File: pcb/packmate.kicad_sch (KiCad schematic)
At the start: 14 parts, among them Q1 2N7002E, SW2 Reset Button, SW3 Left Button, SW4 Right Button, SW6 Wireless On/Off Switch

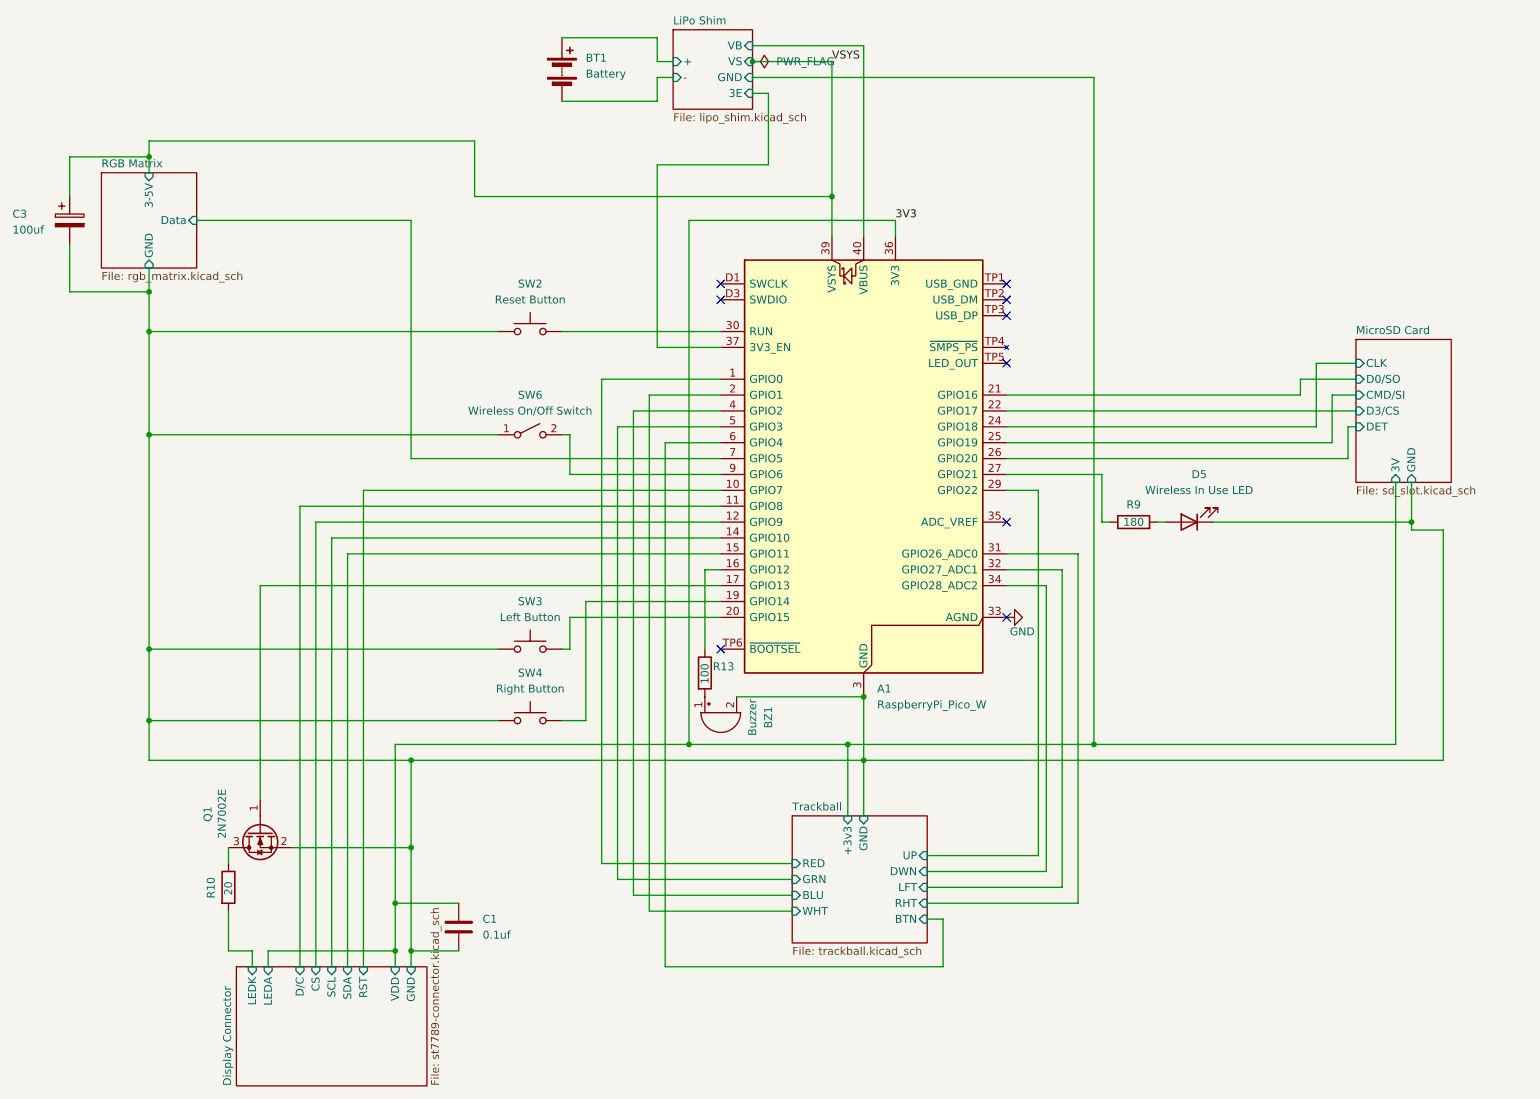
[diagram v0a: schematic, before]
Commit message: Still improving pcb, I learned what a fiducial is today
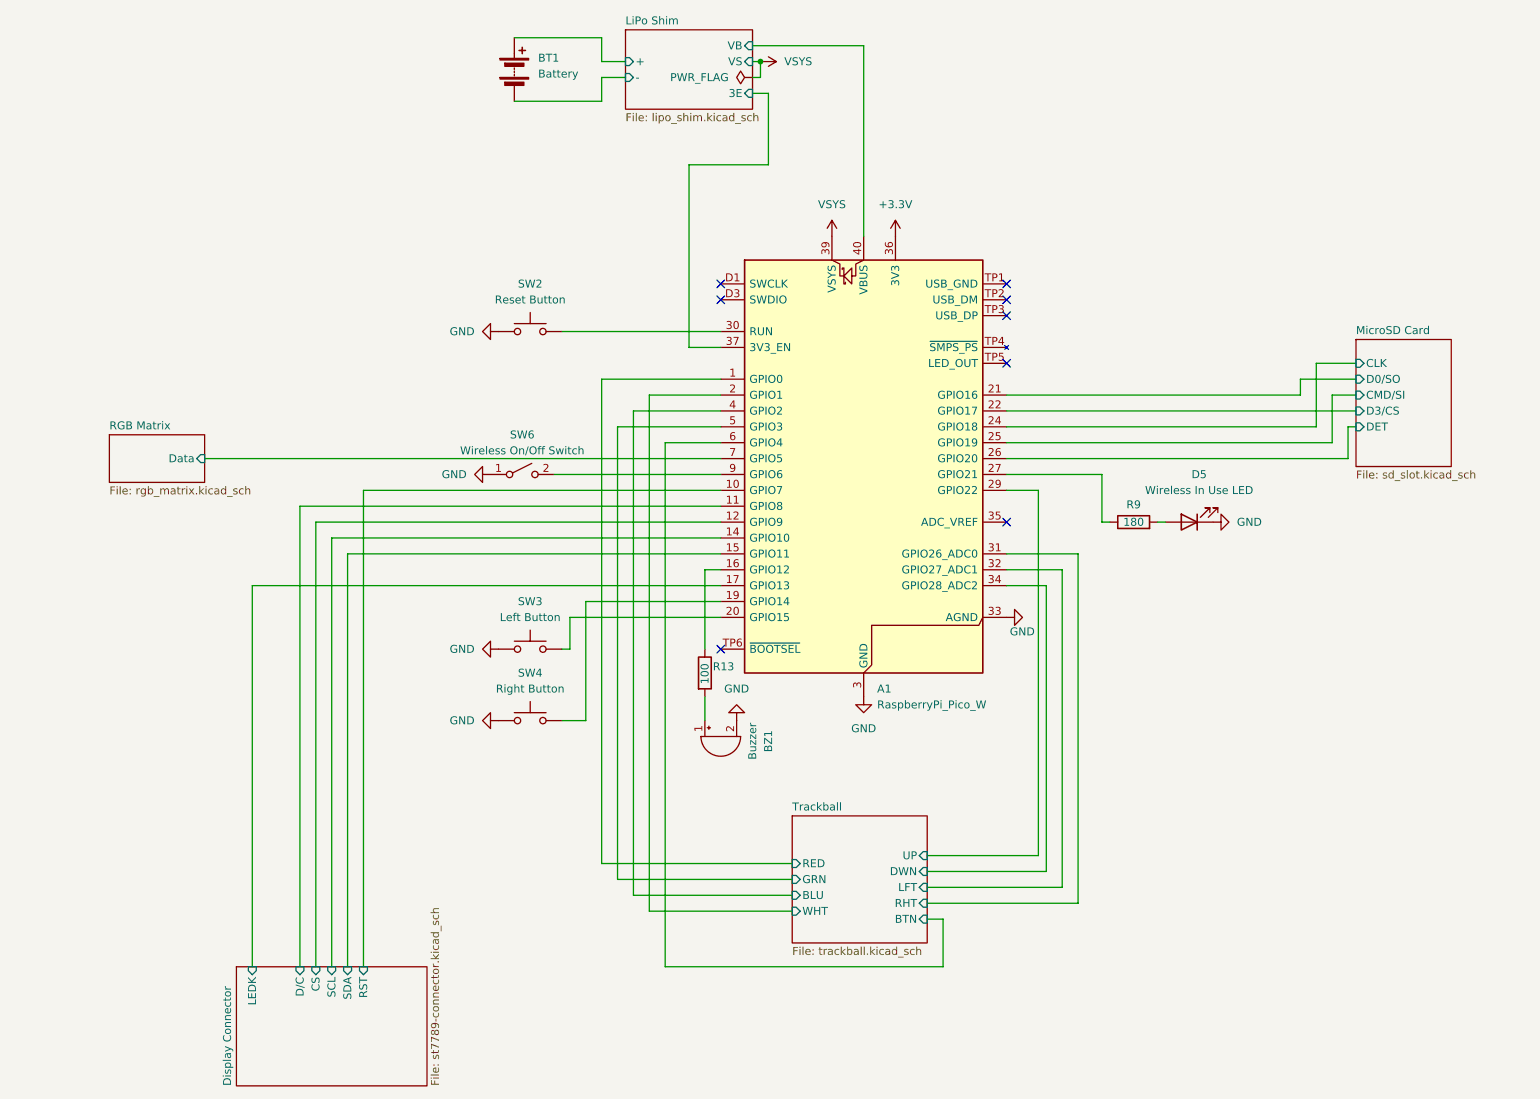
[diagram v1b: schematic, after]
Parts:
- removed C1: 0.1uf, Capacitor_SMD:C_0402_1005Metric, symbol Device:C
- removed C3: 100uf, Capacitor_SMD:CP_Elec_4x5.4, symbol Device:C_Polarized
- removed Q1: 2N7002E, Package_TO_SOT_SMD:SOT-23, symbol Transistor_FET:2N7002E
- removed R10: 20, Resistor_SMD:R_0603_1608Metric, symbol Device:R
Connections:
- net Display Connector/GND is gone; now on net GND: A1.13 (GND), A1.18 (GND), A1.23 (GND), A1.28 (GND), A1.3 (GND), A1.38 (GND), A1.8 (GND), A1.D2 (GND), BZ1.2 (-), D5.1 (K), SW2.1, SW3.1, SW4.1, SW6.1 (A)
- net Display Connector/LEDK: now also A1.17 (GPIO13)
- net 3V3 renamed +3.3V
- no-connect marks 9 -> 8
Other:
- sheet Display Connector ports: added none; removed GND, LEDA, VDD
- sheet LiPo Shim ports: added none; removed GND
- sheet MicroSD Card ports: added none; removed 3V, GND
- sheet RGB Matrix ports: added none; removed 3-5V, GND
- sheet Trackball ports: added none; removed +3v3, GND
- moved on the sheet: BT1, BZ1, SW6
